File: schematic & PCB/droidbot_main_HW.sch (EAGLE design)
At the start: 4 parts

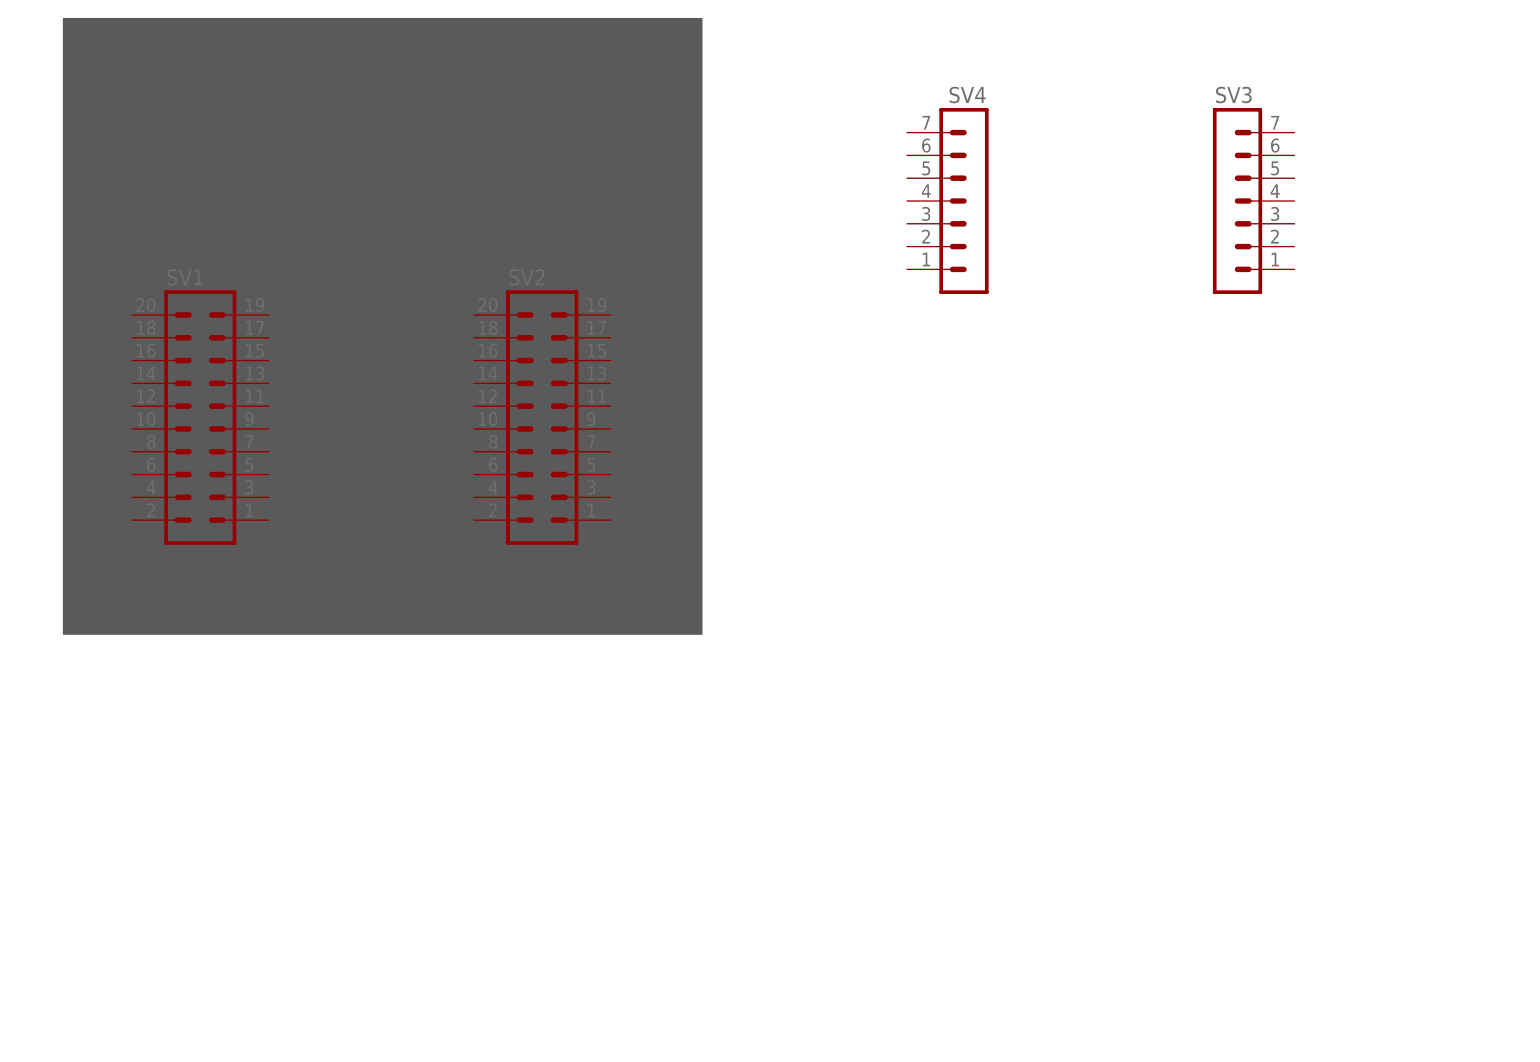
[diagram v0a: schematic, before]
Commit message: work on schematic and pcb
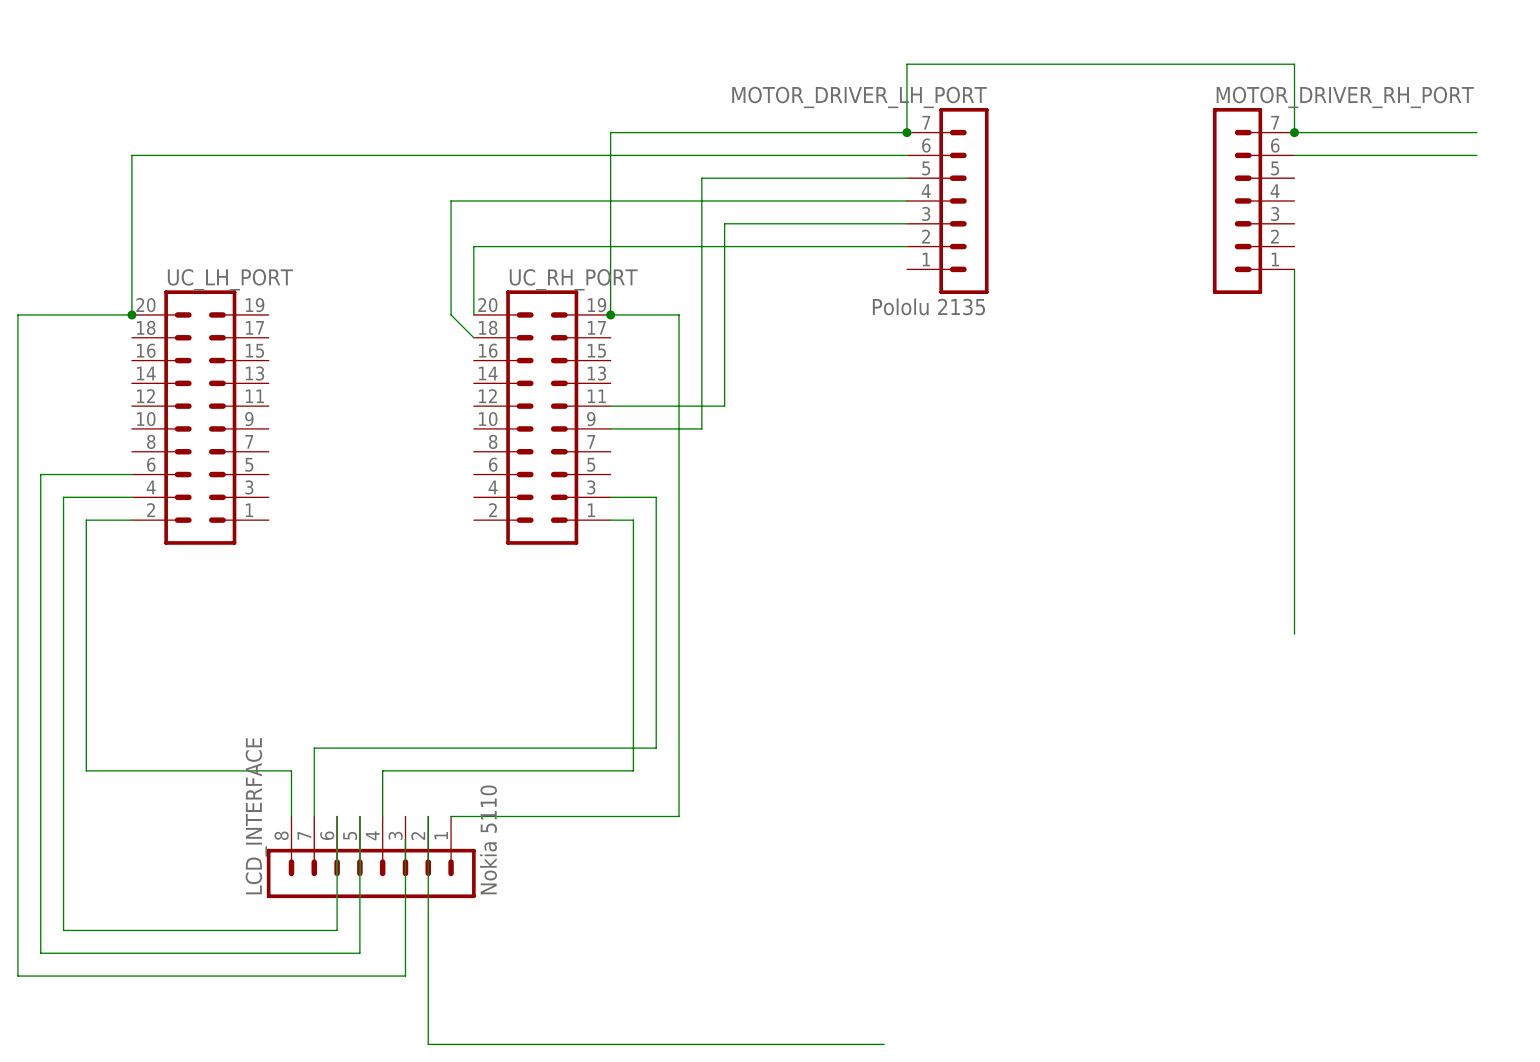
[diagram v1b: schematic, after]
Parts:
- added LCD_INTERFACE: Nokia 5110, con-lstb:MA08-1
- MOTOR_DRIVER_LH_PORT: value (none) -> Pololu 2135
- renumbered SV1 to UC_LH_PORT, SV2 to UC_RH_PORT, SV3 to MOTOR_DRIVER_RH_PORT, SV4 to MOTOR_DRIVER_LH_PORT
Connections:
- new net N$1: LCD_INTERFACE.8, UC_LH_PORT.2
- new net N$10: MOTOR_DRIVER_LH_PORT.4, UC_RH_PORT.18
- new net N$11: MOTOR_DRIVER_LH_PORT.2, UC_RH_PORT.20
- new net N$12: MOTOR_DRIVER_LH_PORT.3, UC_RH_PORT.11
- new net N$13: MOTOR_DRIVER_RH_PORT.6
- new net N$14: MOTOR_DRIVER_RH_PORT.1
- new net N$2: LCD_INTERFACE.7, UC_RH_PORT.3
- new net N$3: LCD_INTERFACE.6, UC_LH_PORT.4
- new net N$4: LCD_INTERFACE.5, UC_LH_PORT.6
- new net N$5: LCD_INTERFACE.4, UC_RH_PORT.1
- new net N$6: MOTOR_DRIVER_LH_PORT.5, UC_RH_PORT.9
- new net N$7: LCD_INTERFACE.2
- new net N$8: MOTOR_DRIVER_LH_PORT.6, UC_LH_PORT.20
- new net N$9: LCD_INTERFACE.1, MOTOR_DRIVER_LH_PORT.7, MOTOR_DRIVER_RH_PORT.7, UC_RH_PORT.19
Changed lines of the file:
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@@
 </classes>
 <parts>
-<part name="SV1" library="con-lstb" deviceset="MA10-2" device=""/>
-<part name="SV2" library="con-lstb" deviceset="MA10-2" device=""/>
-<part name="SV3" library="con-lstb" deviceset="MA07-1" device=""/>
-<part name="SV4" library="con-lstb" deviceset="MA07-1" device=""/>
+<part name="UC_LH_PORT" library="con-lstb" deviceset="MA10-2" device=""/>
+<part name="UC_RH_PORT" library="con-lstb" deviceset="MA10-2" device=""/>
+<part name="MOTOR_DRIVER_RH_PORT" library="con-lstb" deviceset="MA07-1" device=""/>
+<part name="MOTOR_DRIVER_LH_PORT" library="con-lstb" deviceset="MA07-1" device="" value="Pololu 2135"/>
+<part name="LCD_INTERFACE" library="con-lstb" deviceset="MA08-1" device="" value="Nokia 5110"/>
 </parts>
 <sheets>
 <sheet>
 <plain>
-<polygon width="0.1524" layer="97">
-<vertex x="-5.08" y="101.6"/>
-<vertex x="66.04" y="101.6"/>
-<vertex x="66.04" y="33.02"/>
-<vertex x="-5.08" y="33.02"/>
-<vertex x="-5.08" y="35.56"/>
-</polygon>
 <text x="-2.54" y="104.14" size="1.778" layer="93">Tiva C Series
 TM4C123G</text>
-<wire x1="40.64" y1="68.58" x2="40.64" y2="76.2" width="0.1524" layer="100"/>
-<wire x1="40.64" y1="76.2" x2="88.9" y2="76.2" width="0.1524" layer="100"/>
-<wire x1="40.64" y1="66.04" x2="38.1" y2="68.58" width="0.1524" layer="100"/>
-<wire x1="38.1" y1="68.58" x2="38.1" y2="81.28" width="0.1524" layer="100"/>
-<wire x1="38.1" y1="81.28" x2="88.9" y2="81.28" width="0.1524" layer="100"/>
-<wire x1="88.9" y1="78.74" x2="101.6" y2="78.74" width="0.1524" layer="100"/>
-<wire x1="101.6" y1="78.74" x2="101.6" y2="38.1" width="0.1524" layer="100"/>
-<wire x1="101.6" y1="38.1" x2="35.56" y2="38.1" width="0.1524" layer="100"/>
-<wire x1="35.56" y1="38.1" x2="35.56" y2="53.34" width="0.1524" layer="100"/>
-<wire x1="35.56" y1="53.34" x2="40.64" y2="53.34" width="0.1524" layer="100"/>
-<wire x1="40.64" y1="55.88" x2="33.02" y2="55.88" width="0.1524" layer="100"/>
-<wire x1="33.02" y1="55.88" x2="33.02" y2="35.56" width="0.1524" layer="100"/>
-<wire x1="33.02" y1="35.56" x2="104.14" y2="35.56" width="0.1524" layer="100"/>
-<wire x1="104.14" y1="35.56" x2="104.14" y2="83.82" width="0.1524" layer="100"/>
-<wire x1="104.14" y1="83.82" x2="88.9" y2="83.82" width="0.1524" layer="100"/>
 </plain>
 <instances>
-<instance part="SV1" gate="G$1" x="10.16" y="55.88"/>
-<instance part="SV2" gate="G$1" x="48.26" y="55.88"/>
-<instance part="SV3" gate="1" x="124.46" y="81.28"/>
-<instance part="SV4" gate="1" x="96.52" y="81.28" rot="MR0"/>
+<instance part="UC_LH_PORT" gate="G$1" x="10.16" y="55.88"/>
+<instance part="UC_RH_PORT" gate="G$1" x="48.26" y="55.88"/>
+<instance part="MOTOR_DRIVER_RH_PORT" gate="1" x="124.46" y="81.28"/>
+<instance part="MOTOR_DRIVER_LH_PORT" gate="1" x="96.52" y="81.28" rot="MR0"/>
+<instance part="LCD_INTERFACE" gate="1" x="30.48" y="5.08" rot="R90"/>
 </instances>
 <busses>
 </busses>
 <nets>
+<net name="N$1" class="0">
+<segment>
+<pinref part="LCD_INTERFACE" gate="1" pin="8"/>
+<pinref part="UC_LH_PORT" gate="G$1" pin="2"/>
+<wire x1="2.54" y1="45.72" x2="-2.54" y2="45.72" width="0.1524" layer="91"/>
+<wire x1="-2.54" y1="45.72" x2="-2.54" y2="17.78" width="0.1524" layer="91"/>
+<wire x1="-2.54" y1="17.78" x2="20.32" y2="17.78" width="0.1524" layer="91"/>
+<wire x1="20.32" y1="17.78" x2="20.32" y2="12.7" width="0.1524" layer="91"/>
+</segment>
+</net>
+<net name="N$2" class="0">
+<segment>
+<pinref part="LCD_INTERFACE" gate="1" pin="7"/>
+<pinref part="UC_RH_PORT" gate="G$1" pin="3"/>
+<wire x1="55.88" y1="48.26" x2="60.96" y2="48.26" width="0.1524" layer="91"/>
+<wire x1="60.96" y1="48.26" x2="60.96" y2="20.32" width="0.1524" layer="91"/>
+<wire x1="60.96" y1="20.32" x2="22.86" y2="20.32" width="0.1524" layer="91"/>
+<wire x1="22.86" y1="20.32" x2="22.86" y2="12.7" width="0.1524" layer="91"/>
+</segment>
+</net>
+<net name="N$3" class="0">
+<segment>
+<pinref part="LCD_INTERFACE" gate="1" pin="6"/>
+<pinref part="UC_LH_PORT" gate="G$1" pin="4"/>
+<wire x1="2.54" y1="48.26" x2="-5.08" y2="48.26" width="0.1524" layer="91"/>
+<wire x1="-5.08" y1="48.26" x2="-5.08" y2="0" width="0.1524" layer="91"/>
+<wire x1="-5.08" y1="0" x2="25.4" y2="0" width="0.1524" layer="91"/>
+<wire x1="25.4" y1="0" x2="25.4" y2="12.7" width="0.1524" layer="91"/>
+</segment>
+</net>
+<net name="N$4" class="0">
+<segment>
+<pinref part="LCD_INTERFACE" gate="1" pin="5"/>
+<wire x1="27.94" y1="12.7" x2="27.94" y2="-2.54" width="0.1524" layer="91"/>
+<wire x1="27.94" y1="-2.54" x2="-7.62" y2="-2.54" width="0.1524" layer="91"/>
+<pinref part="UC_LH_PORT" gate="G$1" pin="6"/>
+<wire x1="-7.62" y1="-2.54" x2="-7.62" y2="50.8" width="0.1524" layer="91"/>
+<wire x1="-7.62" y1="50.8" x2="2.54" y2="50.8" width="0.1524" layer="91"/>
+</segment>
+</net>
+<net name="N$5" class="0">
+<segment>
+<pinref part="LCD_INTERFACE" gate="1" pin="4"/>
+<pinref part="UC_RH_PORT" gate="G$1" pin="1"/>
+<wire x1="55.88" y1="45.72" x2="58.42" y2="45.72" width="0.1524" layer="91"/>
+<wire x1="58.42" y1="45.72" x2="58.42" y2="17.78" width="0.1524" layer="91"/>
+<wire x1="58.42" y1="17.78" x2="30.48" y2="17.78" width="0.1524" layer="91"/>
+<wire x1="30.48" y1="17.78" x2="30.48" y2="12.7" width="0.1524" layer="91"/>
+</segment>
+</net>
+<net name="N$7" class="0">
+<segment>
+<pinref part="LCD_INTERFACE" gate="1" pin="2"/>
+<wire x1="35.56" y1="12.7" x2="35.56" y2="-12.7" width="0.1524" layer="91"/>
+<wire x1="35.56" y1="-12.7" x2="86.36" y2="-12.7" width="0.1524" layer="91"/>
+</segment>
+</net>
+<net name="N$9" class="0">
+<segment>
+<pinref part="MOTOR_DRIVER_LH_PORT" gate="1" pin="7"/>
+<pinref part="UC_RH_PORT" gate="G$1" pin="19"/>
+<wire x1="88.9" y1="88.9" x2="55.88" y2="88.9" width="0.1524" layer="91"/>
+<wire x1="55.88" y1="88.9" x2="55.88" y2="68.58" width="0.1524" layer="91"/>
+<wire x1="55.88" y1="68.58" x2="63.5" y2="68.58" width="0.1524" layer="91"/>
+<pinref part="LCD_INTERFACE" gate="1" pin="1"/>
+<wire x1="63.5" y1="68.58" x2="63.5" y2="12.7" width="0.1524" layer="91"/>
+<wire x1="63.5" y1="12.7" x2="38.1" y2="12.7" width="0.1524" layer="91"/>
+<junction x="55.88" y="68.58"/>
+<wire x1="88.9" y1="88.9" x2="88.9" y2="96.52" width="0.1524" layer="91"/>
+<junction x="88.9" y="88.9"/>
+<wire x1="88.9" y1="96.52" x2="132.08" y2="96.52" width="0.1524" layer="91"/>
+<pinref part="MOTOR_DRIVER_RH_PORT" gate="1" pin="7"/>
+<wire x1="132.08" y1="96.52" x2="132.08" y2="88.9" width="0.1524" layer="91"/>
+<wire x1="132.08" y1="88.9" x2="152.4" y2="88.9" width="0.1524" layer="91"/>
+<junction x="132.08" y="88.9"/>
+</segment>
+</net>
+<net name="N$10" class="0">
+<segment>
+<pinref part="MOTOR_DRIVER_LH_PORT" gate="1" pin="4"/>
+<wire x1="88.9" y1="81.28" x2="38.1" y2="81.28" width="0.1524" layer="91"/>
+<pinref part="UC_RH_PORT" gate="G$1" pin="18"/>
+<wire x1="38.1" y1="81.28" x2="38.1" y2="68.58" width="0.1524" layer="91"/>
+<wire x1="38.1" y1="68.58" x2="40.64" y2="66.04" width="0.1524" layer="91"/>
+</segment>
+</net>
+<net name="N$11" class="0">
+<segment>
+<pinref part="MOTOR_DRIVER_LH_PORT" gate="1" pin="2"/>
+<pinref part="UC_RH_PORT" gate="G$1" pin="20"/>
+<wire x1="88.9" y1="76.2" x2="40.64" y2="76.2" width="0.1524" layer="91"/>
+<wire x1="40.64" y1="76.2" x2="40.64" y2="68.58" width="0.1524" layer="91"/>
+</segment>
+</net>
+<net name="N$8" class="0">
+<segment>
+<wire x1="33.02" y1="10.16" x2="33.02" y2="-5.08" width="0.1524" layer="91"/>
+<wire x1="33.02" y1="-5.08" x2="-10.16" y2="-5.08" width="0.1524" layer="91"/>
+<pinref part="UC_LH_PORT" gate="G$1" pin="20"/>
+<wire x1="-10.16" y1="-5.08" x2="-10.16" y2="68.58" width="0.1524" layer="91"/>
+<wire x1="-10.16" y1="68.58" x2="2.54" y2="68.58" width="0.1524" layer="91"/>
+<pinref part="MOTOR_DRIVER_LH_PORT" gate="1" pin="6"/>
+<wire x1="88.9" y1="86.36" x2="2.54" y2="86.36" width="0.1524" layer="91"/>
+<wire x1="2.54" y1="86.36" x2="2.54" y2="68.58" width="0.1524" layer="91"/>
+<junction x="2.54" y="68.58"/>
+</segment>
+</net>
+<net name="N$6" class="0">
+<segment>
+<pinref part="MOTOR_DRIVER_LH_PORT" gate="1" pin="5"/>
+<wire x1="88.9" y1="83.82" x2="66.04" y2="83.82" width="0.1524" layer="91"/>
+<wire x1="66.04" y1="83.82" x2="66.04" y2="55.88" width="0.1524" layer="91"/>
+<pinref part="UC_RH_PORT" gate="G$1" pin="9"/>
+<wire x1="66.04" y1="55.88" x2="55.88" y2="55.88" width="0.1524" layer="91"/>
+</segment>
+</net>
+<net name="N$12" class="0">
+<segment>
+<pinref part="MOTOR_DRIVER_LH_PORT" gate="1" pin="3"/>
+<wire x1="88.9" y1="78.74" x2="68.58" y2="78.74" width="0.1524" layer="91"/>
+<wire x1="68.58" y1="78.74" x2="68.58" y2="58.42" width="0.1524" layer="91"/>
+<pinref part="UC_RH_PORT" gate="G$1" pin="11"/>
+<wire x1="68.58" y1="58.42" x2="55.88" y2="58.42" width="0.1524" layer="91"/>
+</segment>
+</net>
+<net name="N$13" class="0">
+<segment>
+<pinref part="MOTOR_DRIVER_RH_PORT" gate="1" pin="6"/>
+<wire x1="132.08" y1="86.36" x2="152.4" y2="86.36" width="0.1524" layer="91"/>
+</segment>
+</net>
+<net name="N$14" class="0">
+<segment>
+<pinref part="MOTOR_DRIVER_RH_PORT" gate="1" pin="1"/>
+<wire x1="132.08" y1="73.66" x2="132.08" y2="33.02" width="0.1524" layer="91"/>
+</segment>
+</net>
 </nets>
 </sheet>
